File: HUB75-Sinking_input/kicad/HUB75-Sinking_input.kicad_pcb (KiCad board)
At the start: 2 copper layers, 85 x 56 mm, 81 parts, among them J1 Conn_01x03_Male, J10 Conn_01x03_Male, J11 Conn_01x03_Male, J12 Conn_01x03_Male, J2 Conn_01x03_Male, J3 Conn_01x03_Male, J4 Conn_01x03_Male, J5 Conn_01x03_Male, J6 Conn_01x03_Male, J7 Conn_01x03_Male, J8 Conn_01x03_Male, J9 Conn_01x03_Male, Q1 AO3401A, Q10 2N7002, Q11 2N7002, Q12 2N7002, Q13 2N7002, Q14 2N7002, Q2 2N7002, Q3 2N7002, Q4 2N7002, Q5 2N7002, Q6 2N7002, Q7 2N7002, Q8 2N7002, Q9 2N7002, U1 CL2N8-G, U2 LTV-827, U3 LTV-827, U4 LTV-827, U5 LTV-827, U6 LTV-827, U7 LTV-827

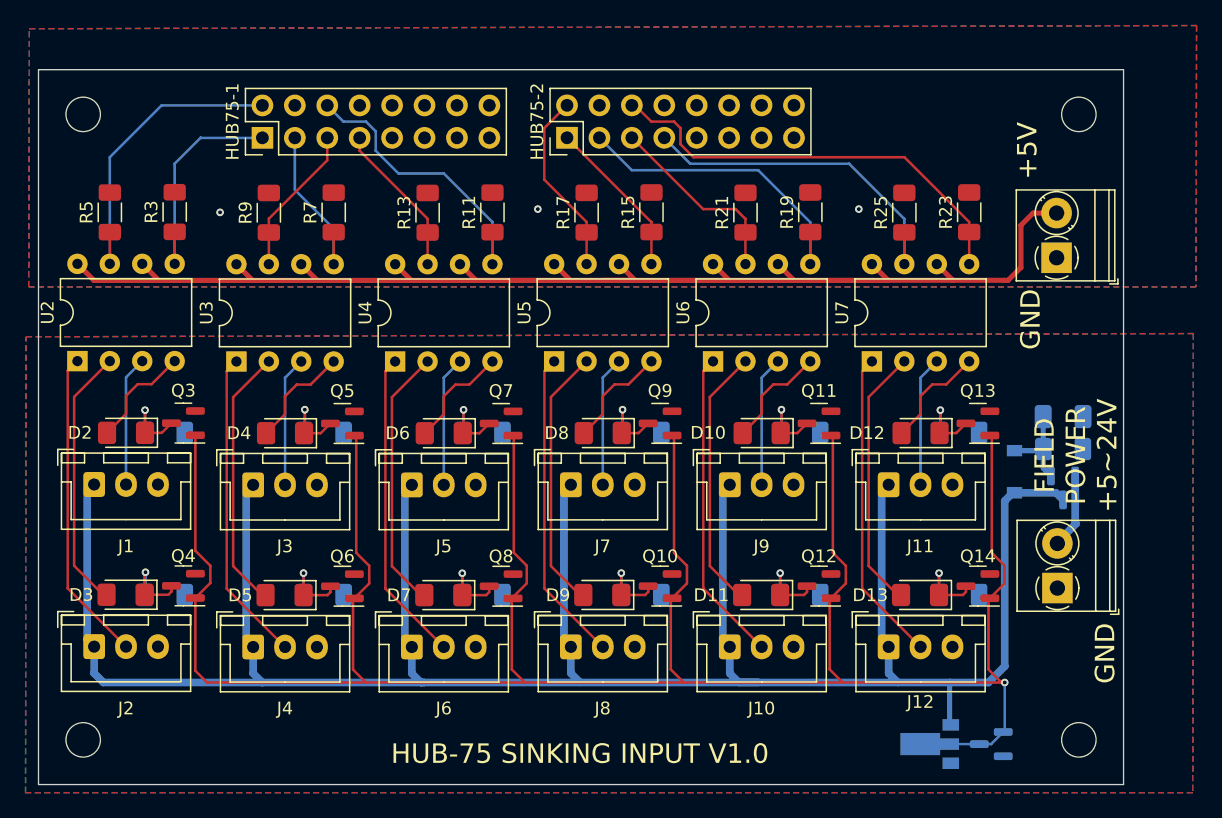
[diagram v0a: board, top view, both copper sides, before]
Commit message: Regenerated
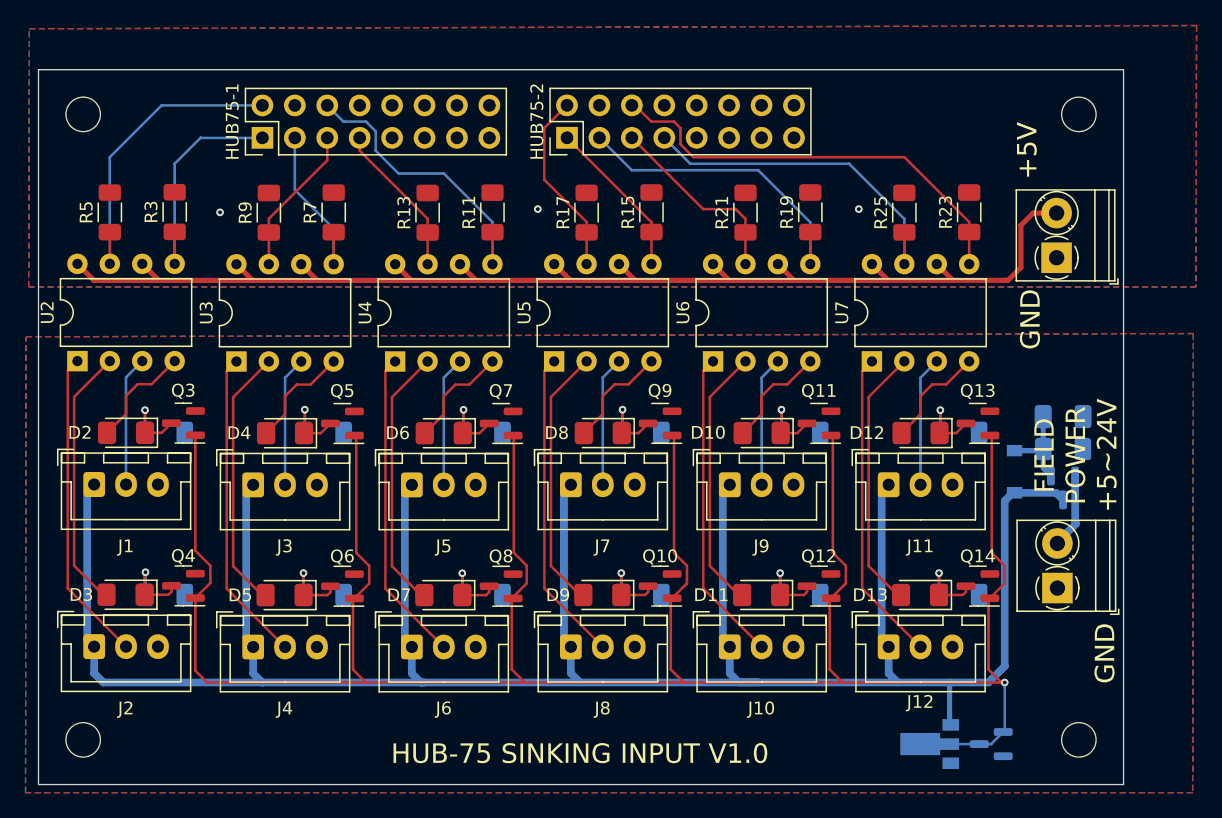
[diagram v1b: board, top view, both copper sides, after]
